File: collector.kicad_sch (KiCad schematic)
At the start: 2 parts, among them U14 CD74HCT32E

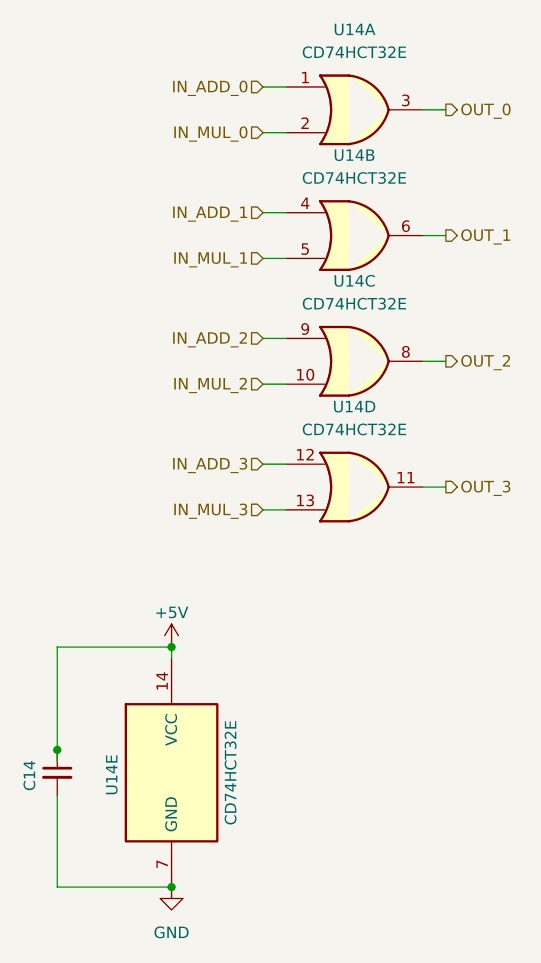
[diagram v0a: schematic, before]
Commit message: fix: 0 error 0 warning
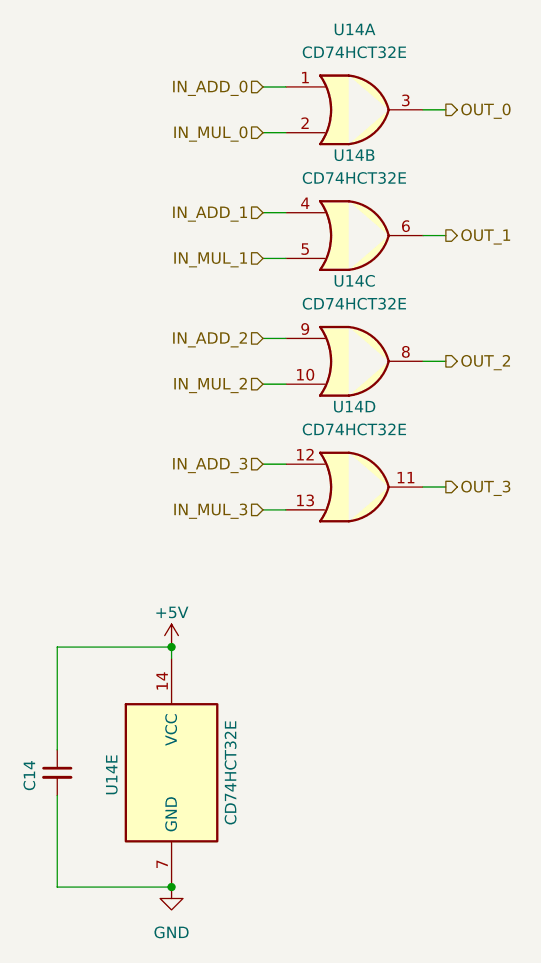
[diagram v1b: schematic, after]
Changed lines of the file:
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@@
 	(paper "A4")
-	(junction
-		(at 58.42 124.46)
-		(diameter 0)
-		(color 0 0 0 0)
-	)
 	(junction
 		(at 71.12 139.7)
@@
 		(pts
 			(xy 81.28 50.8) (xy 83.82 50.8)
-		)
-		(stroke
-			(width 0)
-			(type default)
-		)
-	)
-	(wire
-		(pts
-			(xy 58.42 124.46) (xy 58.42 113.03)
-		)
-		(stroke
-			(width 0)
-			(type default)
-		)
-	)
-	(wire
-		(pts
-			(xy 58.42 125.73) (xy 58.42 124.46)
 		)
 		(stroke
@@
 		)
 		(stroke
+			(width 0)
+			(type default)
+		)
+	)
+	(wire
+		(pts
+			(xy 58.42 113.03) (xy 58.42 124.46)
+		)
+		(stroke
